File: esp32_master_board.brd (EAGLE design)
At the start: 65 x 35 mm, 66 parts, among them IC1 SN74HC138PW, IC2 MAX17502EATB+T, IC3 WS2812B, IC4 WS2812B, SW1 B3U-1000P-2P-SMD

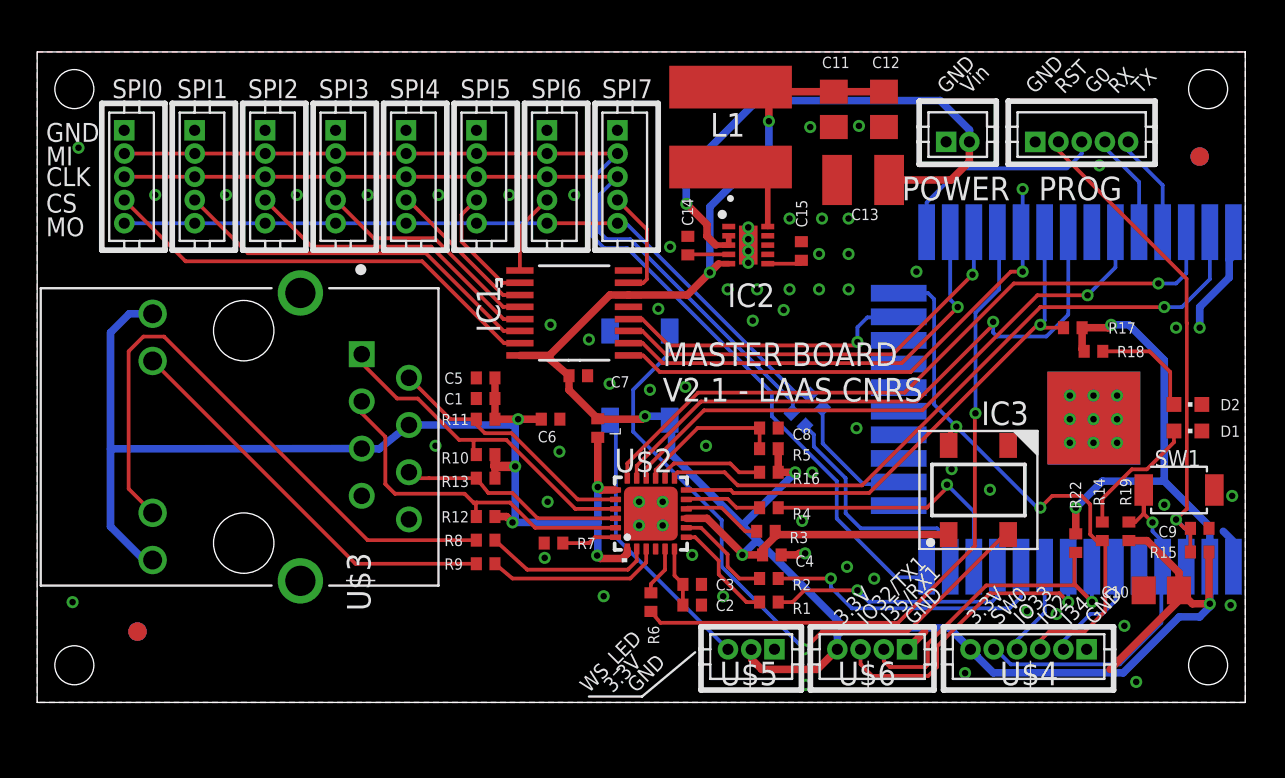
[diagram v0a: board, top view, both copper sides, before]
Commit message: Fusion Model
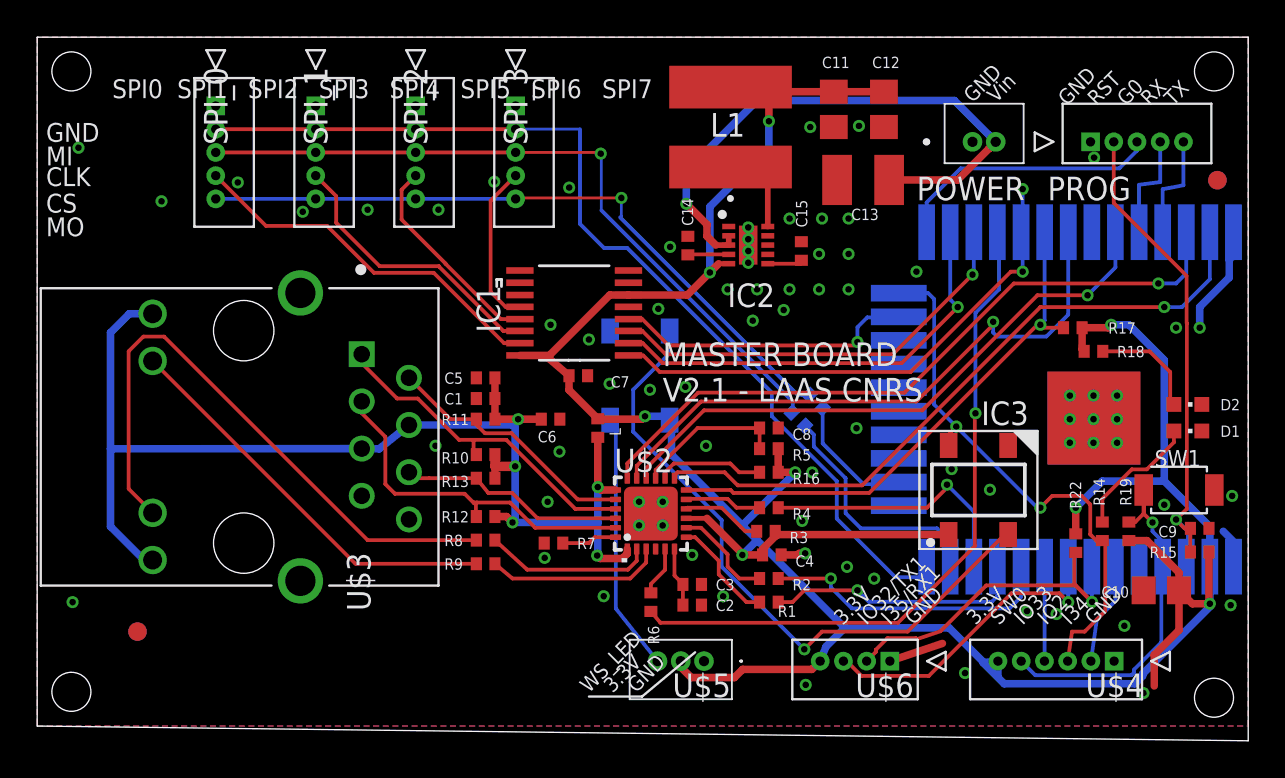
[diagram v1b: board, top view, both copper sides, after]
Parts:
- removed SPI_4, SPI_5, SPI_6, SPI_7: DF13-5P-1.25DSA, con-hirose-df13:DF13-5P-1.25DSA
- POWER: value DF13-2P-1.25DSA -> 53047-0210; device con-hirose-df13:DF13-2P-1.25DSA -> 53047-0210:530470210
- PROG, SPI_0, SPI_1, SPI_2, SPI_3: value DF13-5P-1.25DSA -> 53047-0510; device con-hirose-df13:DF13-5P-1.25DSA -> 53047-0510:530470510
- U$4: value DF13-6P-1.25DSA -> 53047-0610; device con-hirose-df13:DF13-6P-1.25DSA -> 53047-0610:530470610
- U$5: value DF13-3P-1.25DSA -> 53047-0310; device con-hirose-df13:DF13-3P-1.25DSA -> 53047-0310:530470310
- U$6: value DF13-4P-1.25DSA -> 530470410; device con-hirose-df13:DF13-4P-1.25DSA -> 530470410:530470410
- moved SPI_3 10.4 mm to (25.7, 32.1)
- moved SPI_2 8.95 mm to (20.4, 32.1)
- moved SPI_1 7.54 mm to (15.0, 32.1)
- moved SPI_0 6.22 mm to (9.61, 32.1)
- moved U$4 4.65 mm to (57.9, 2.22)
- moved U$5 2.62 mm to (35.9, 2.22)
- moved REF2 1.59 mm to (63.5, 28.1)
- moved REF4 1.59 mm to (63.5, 28.1)
- moved U$6 1.14 mm to (45.9, 2.22)
- moved POWER 0.79 mm to (50.3, 30.2)
- moved PROG 0.48 mm to (56.7, 30.2)
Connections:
- net BOOT_MODE: now also PROG.3; no longer PROG.P$3
- net GND: now also POWER.1, PROG.1, SPI_0.1, SPI_1.1, SPI_2.1, SPI_3.1, U$4.1, U$5.1, U$6.1; no longer POWER.P$1, PROG.P$1, SPI_0.P$1, SPI_1.P$1, SPI_2.P$1, SPI_3.P$1, SPI_4.P$1, SPI_5.P$1, SPI_6.P$1, SPI_7.P$1, U$4.P$1, U$5.P$1, U$6.P$1
- net I34: now also U$4.2; no longer U$4.P$2
- net I35_RX1: now also U$6.2; no longer U$6.P$2
- net IO2: now also U$4.3; no longer U$4.P$3
- net IO32_TX1: now also U$6.3; no longer U$6.P$3
- net IO33: now also U$4.4; no longer U$4.P$4
- net N$25: now also POWER.2; no longer POWER.P$2
- net RST: now also PROG.2; no longer PROG.P$2
- net RX: now also PROG.4; no longer PROG.P$4
- net SPI_CLK: now also SPI_0.3, SPI_1.3, SPI_2.3, SPI_3.3; no longer SPI_0.P$3, SPI_1.P$3, SPI_2.P$3, SPI_3.P$3, SPI_4.P$3, SPI_5.P$3, SPI_6.P$3, SPI_7.P$3
- net SPI_CS0: now also SPI_0.4; no longer SPI_0.P$4
- net SPI_CS1: now also SPI_1.4; no longer SPI_1.P$4
- net SPI_CS2: now also SPI_2.4; no longer SPI_2.P$4
- net SPI_CS3: now also SPI_3.4; no longer SPI_3.P$4
- net SPI_CS4: no longer SPI_4.P$4
- net SPI_CS5: no longer SPI_5.P$4
- net SPI_CS6: no longer SPI_6.P$4
- net SPI_CS7: no longer SPI_7.P$4
- net SPI_MISO: now also SPI_0.2, SPI_1.2, SPI_2.2, SPI_3.2; no longer SPI_0.P$2, SPI_1.P$2, SPI_2.P$2, SPI_3.P$2, SPI_4.P$2, SPI_5.P$2, SPI_6.P$2, SPI_7.P$2
- net SPI_MOSI: now also SPI_0.5, SPI_1.5, SPI_2.5, SPI_3.5; no longer SPI_0.P$5, SPI_1.P$5, SPI_2.P$5, SPI_3.P$5, SPI_4.P$5, SPI_5.P$5, SPI_6.P$5, SPI_7.P$5
- net SW0: now also U$4.5; no longer U$4.P$5
- net TX: now also PROG.5; no longer PROG.P$5
- net VCC: now also U$4.6, U$5.2, U$6.4; no longer U$4.P$6, U$5.P$2, U$6.P$4
- net WSLED_OUT: now also U$5.3; no longer U$5.P$3
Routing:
- net SPI_CS4: track 8.24 -> 0.00 mm
- net VCC: track 153.5 -> 160.2 mm
- net SPI_CS5: track 6.65 -> 0.00 mm
- net SPI_CS7: track 5.99 -> 0.00 mm
- net SPI_MISO: track 59.6 -> 53.6 mm
- net SPI_CLK: track 44.7 -> 39.0 mm, vias 0 -> 1
- net SPI_CS1: track 20.4 -> 15.3 mm
- net SPI_CS2: track 16.4 -> 11.3 mm
- net SPI_CS6: track 4.40 -> 0.00 mm
- net SPI_CS0: track 24.5 -> 20.1 mm
- net SPI_MOSI: track 40.7 -> 37.1 mm, vias 0 -> 1
- net SPI_CS3: track 12.3 -> 8.72 mm
- net BOOT_MODE: track 11.7 -> 14.5 mm
- net N$25: track 29.7 -> 31.6 mm
- net GND: track 21.5 -> 23.2 mm
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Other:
- board size 65 x 35 mm -> 65.2 x 37.9 mm
